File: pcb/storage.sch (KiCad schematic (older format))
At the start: 31 parts, among them Q300 IRLML6402, Q302 2SK3018, U100 MCIMX7S5EVM08SC, U300 ADP123, U301 W25Q16BV

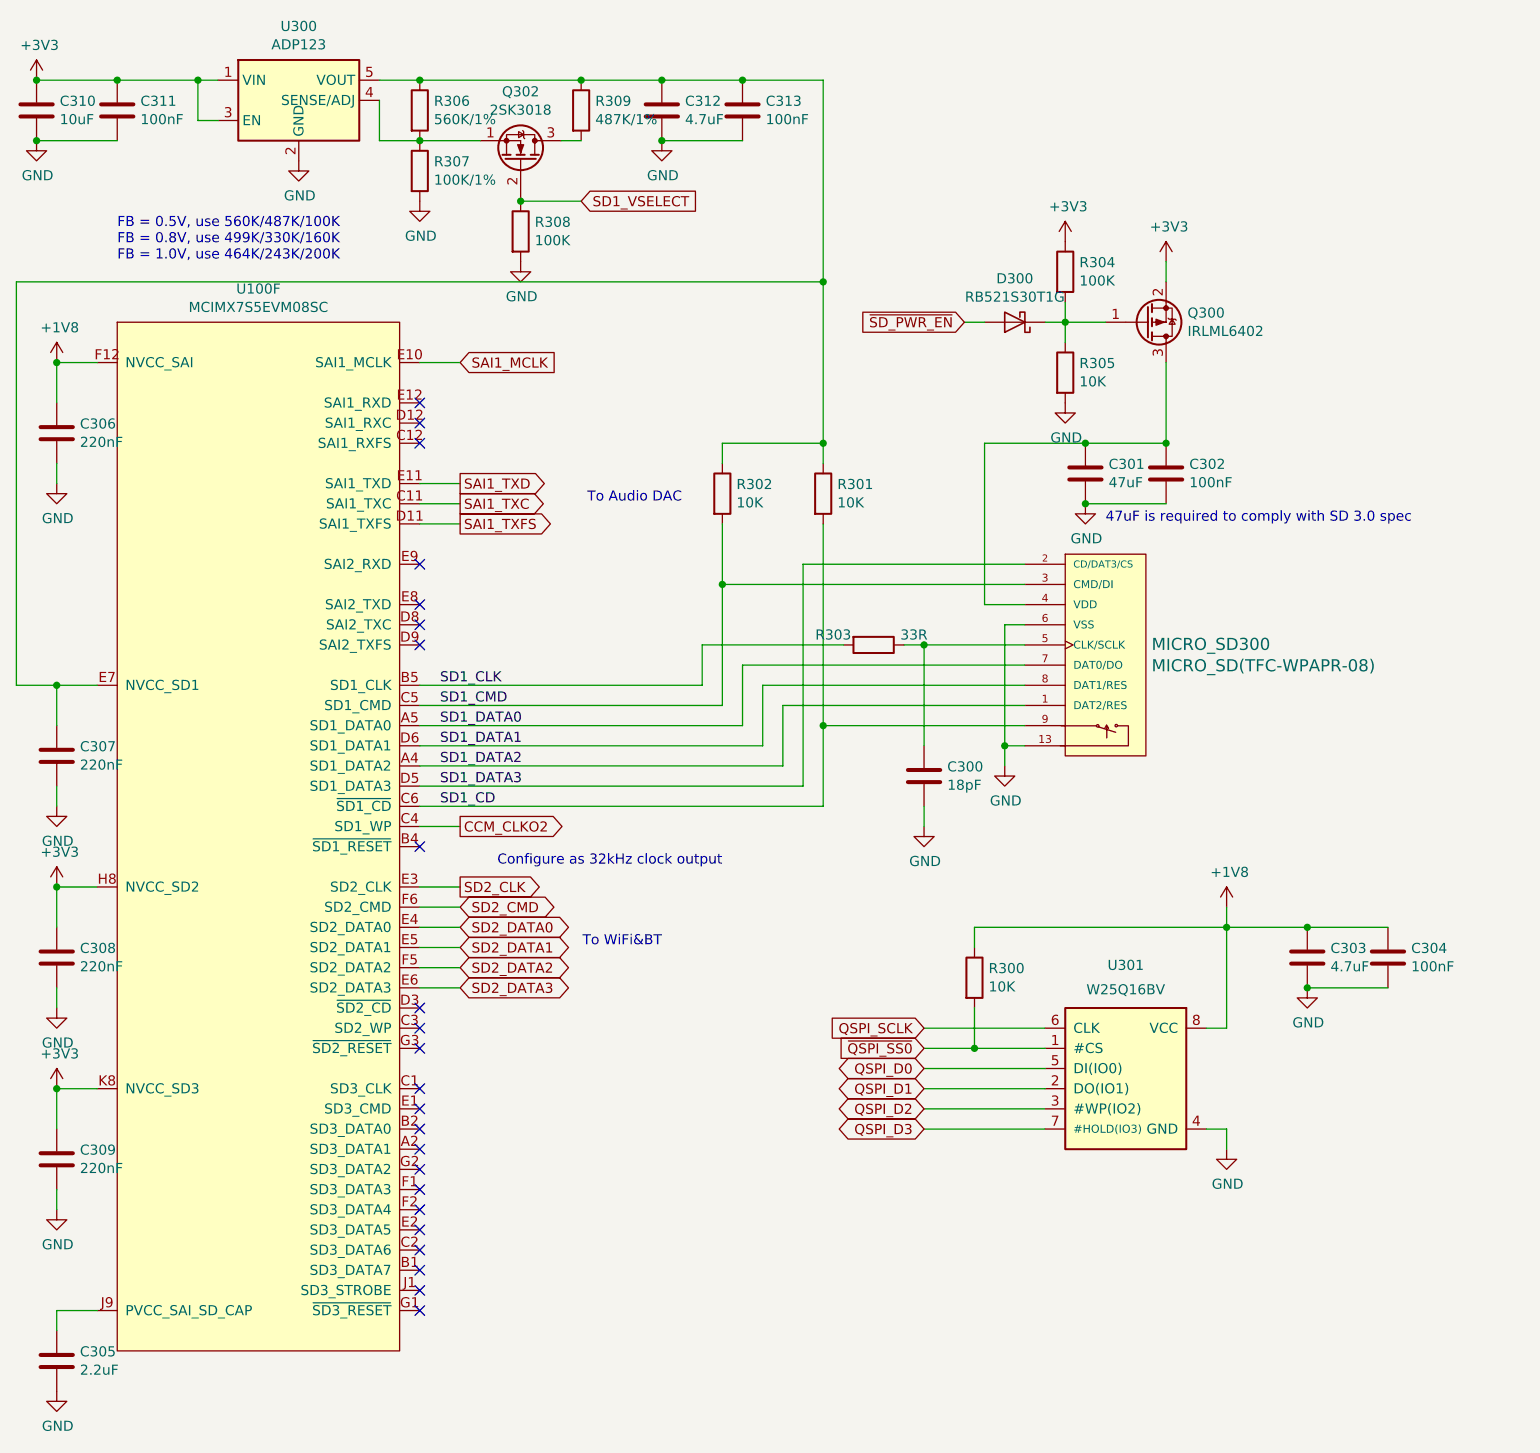
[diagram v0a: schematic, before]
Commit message: pcb: rev 0.1
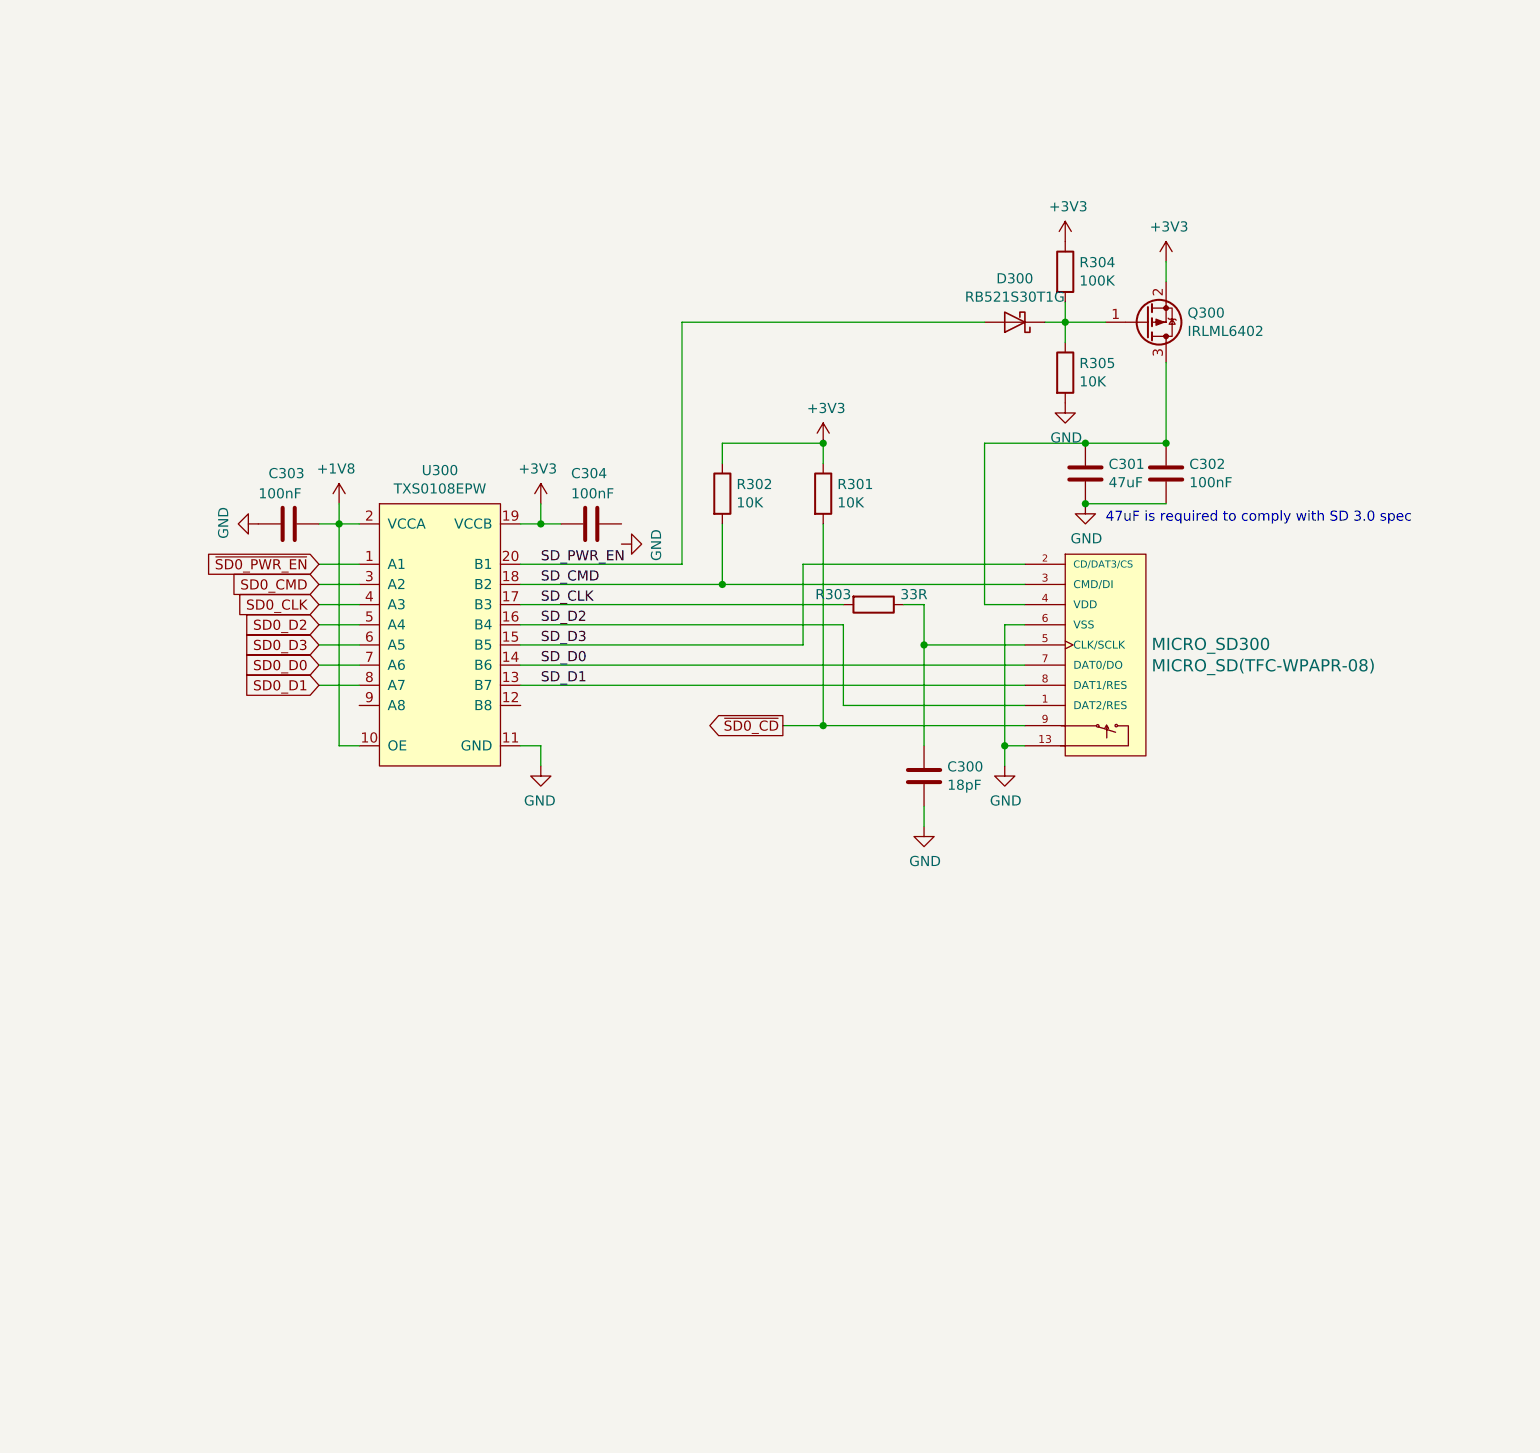
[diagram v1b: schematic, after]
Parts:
- removed C305: 2.2uF, Capacitor_SMD:C_0402_1005Metric, symbol Device:C
- removed C306, C307, C308, C309: 220nF, Capacitor_SMD:C_0402_1005Metric, symbol Device:C
- removed C310: 10uF, Capacitor_SMD:C_0603_1608Metric, symbol Device:C
- removed C311, C313: 100nF, Capacitor_SMD:C_0402_1005Metric, symbol Device:C
- removed C312: 4.7uF, Capacitor_SMD:C_0603_1608Metric, symbol Device:C
- removed Q302: 2SK3018, Package_TO_SOT_SMD:SOT-23, symbol Device:Q_NMOS_SGD
- removed R300: 10K, Resistor_SMD:R_0603_1608Metric, symbol Device:R
- removed R306: 560K/1%, Resistor_SMD:R_0603_1608Metric, symbol Device:R
- removed R307: 100K/1%, Resistor_SMD:R_0603_1608Metric, symbol Device:R
- removed R308: 100K, Resistor_SMD:R_0603_1608Metric, symbol Device:R
- removed R309: 487K/1%, Resistor_SMD:R_0603_1608Metric, symbol Device:R
- removed U100: MCIMX7S5EVM08SC, footprints:BGA-541_25x25_19.0x19.0mm, symbol symbols:MCIMX7S5EVM08SC
- removed U300: ADP123, Package_TO_SOT_SMD:TSOT-23-5, symbol Regulator_Linear:ADP7142AUJZ
- removed U301: W25Q16BV, Package_SON:WSON-8-1EP_6x5mm_P1.27mm_EP3.4x4mm, symbol symbols:W25Q16BV
- added U300: TXS0108EPW, Package_SO:TSSOP-20_4.4x6.5mm_P0.65mm, symbol symbols:TXS0108EPW
- C303: value 4.7uF -> 100nF; footprint Capacitor_SMD:C_0603_1608Metric -> Capacitor_SMD:C_0402_1005Metric
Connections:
- net +1V8: now also U300.10 (OE), U300.2 (VCCA); no longer C304.1
- net +3V3: now also C304.2, R301.1, R302.1, U300.19 (VCCB)
- net GND: now also U300.11 (GND); no longer C304.2
- net SD1_CD renamed ~SD0_CD
- net SD1_CLK renamed SD_CLK
- net SD_CLK: now also U300.17 (B3)
- net SD1_CMD renamed SD_CMD
- net SD_CMD: now also U300.18 (B2)
- net SD1_DATA0 renamed SD_D0
- net SD_D0: now also U300.14 (B6)
- net SD1_DATA1 renamed SD_D1
- net SD_D1: now also U300.13 (B7)
- net SD1_DATA2 renamed SD_D2
- net SD_D2: now also U300.16 (B4)
- net SD1_DATA3 renamed SD_D3
- net SD_D3: now also U300.15 (B5)
- net ~SD_PWR_EN renamed SD_PWR_EN
- net SD_PWR_EN: now also U300.20 (B1)
- new net SD0_CLK: U300.4 (A3)
- new net SD0_CMD: U300.3 (A2)
- new net SD0_D0: U300.7 (A6)
- new net SD0_D1: U300.8 (A7)
- new net SD0_D2: U300.5 (A4)
- new net SD0_D3: U300.6 (A5)
- new net ~SD0_PWR_EN: U300.1 (A1)
- no-connect marks 23 -> 0
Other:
- note removed: "Configure as 32kHz clock output"
- note removed: "FB = 0.5V, use 560K/487K/100K\nFB = 0.8V, use 499K/330K/160K\nFB = 1.0V, use 464K/243K/200K"
- note removed: "To Audio DAC\n"
- note removed: "To WiFi&BT"
- moved on the sheet: R303
